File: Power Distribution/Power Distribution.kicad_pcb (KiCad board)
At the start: 16 copper layers, 61 x 88 mm, 28 parts, among them IC3 PCM5102 Audio Stereo DAC

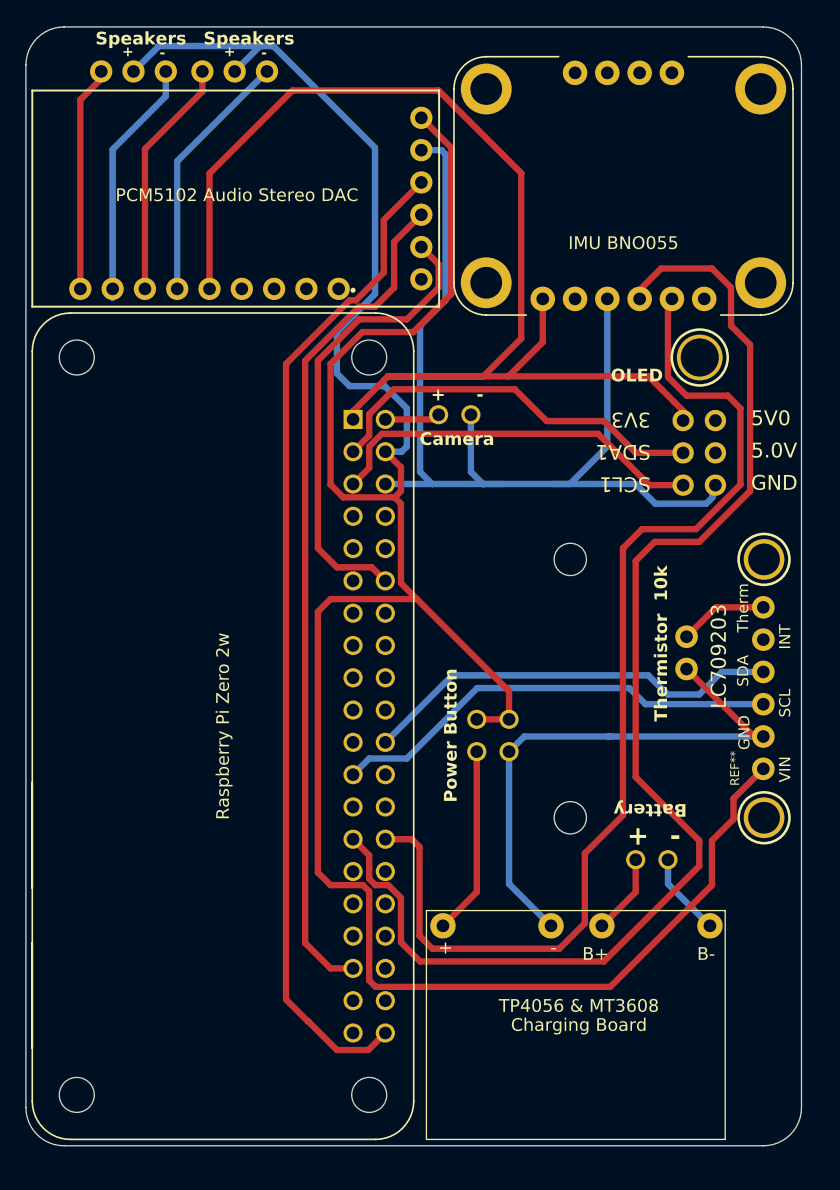
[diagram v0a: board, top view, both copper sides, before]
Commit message: PCB
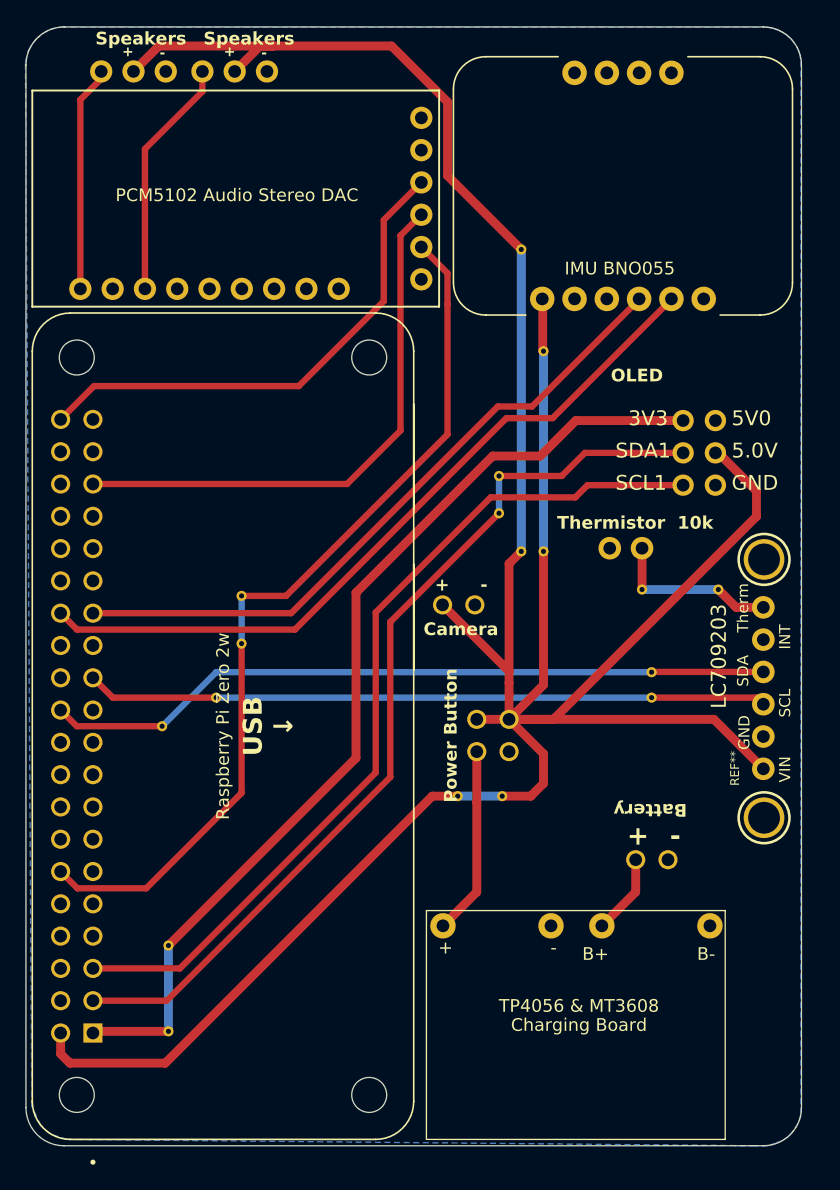
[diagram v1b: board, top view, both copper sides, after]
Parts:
- removed the REF** at (260.5, 100.0)
- removed UNK_HOLE_0: , LC709203F:dummyfp0
- removed UNK_HOLE_1: , LC709203F:dummyfp1
- added ?: , , F.Cu at (248.2, 99.5)
- added ?: , , F.Cu at (224.5, 118.8)
- added ?: , , F.Cu at (256.0, 118.2)
- added ?: , , F.Cu at (245.0, 134.5)
- added ?: , , F.Cu at (222.5, 126.8)
- added ?: , , F.Cu at (241.5, 134.5)
- added ?: , , F.Cu at (218.8, 146.2)
- added ?: , , F.Cu at (246.5, 91.5)
- added ?: , , F.Cu at (218.8, 153.0)
- added ?: , , F.Cu at (246.5, 115.2)
- added ?: , , F.Cu at (218.2, 129.0)
- added ?: , , F.Cu at (248.2, 115.2)
- added ?: , , F.Cu at (244.8, 112.2)
- added ?: , , F.Cu at (244.8, 109.3)
- added ?: , , F.Cu at (224.5, 122.5)
- added ?: , , F.Cu at (262.0, 118.2)
- added ?: , , F.Cu at (256.8, 124.8)
- added ?: , , F.Cu at (256.8, 126.8)
- moved ? 15.0 mm to (242.8, 119.5)
- moved ? 15.0 mm to (240.3, 119.5)
- moved ? 11.3 mm to (253.5, 115.0), turned to -90 degrees
- moved ? 7.79 mm to (256.0, 115.0), turned to -90 degrees
- moved G*** 0.84 mm to (219.8, 157.4)
- turned REF** to 90 degrees
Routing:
- net (no net): track 1048.8 -> 905.4 mm
- added copper zone on B.Cu, net (none)
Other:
- board text added: "USB ↓"
